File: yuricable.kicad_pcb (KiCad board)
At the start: 2 copper layers, 66.2 x 29.2 mm, 34 parts, among them U1 FlipperZero

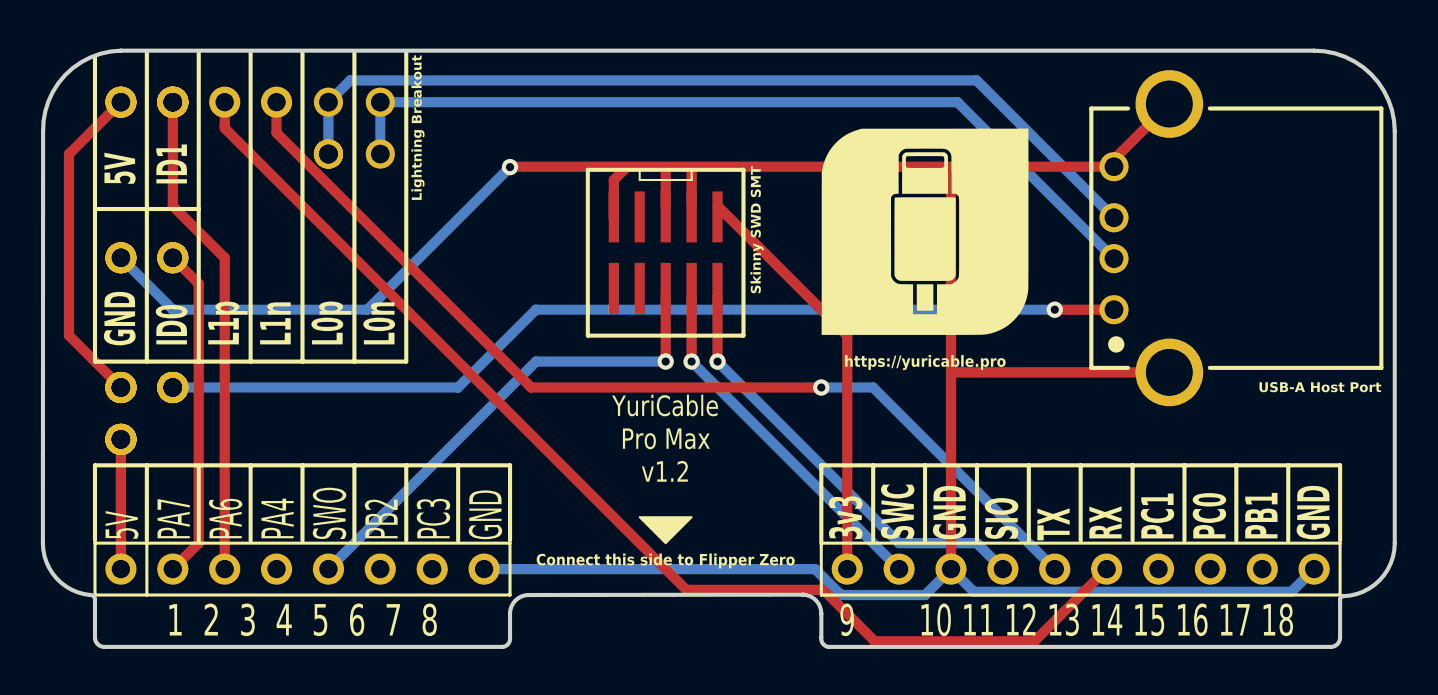
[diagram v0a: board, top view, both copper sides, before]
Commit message: v1.3
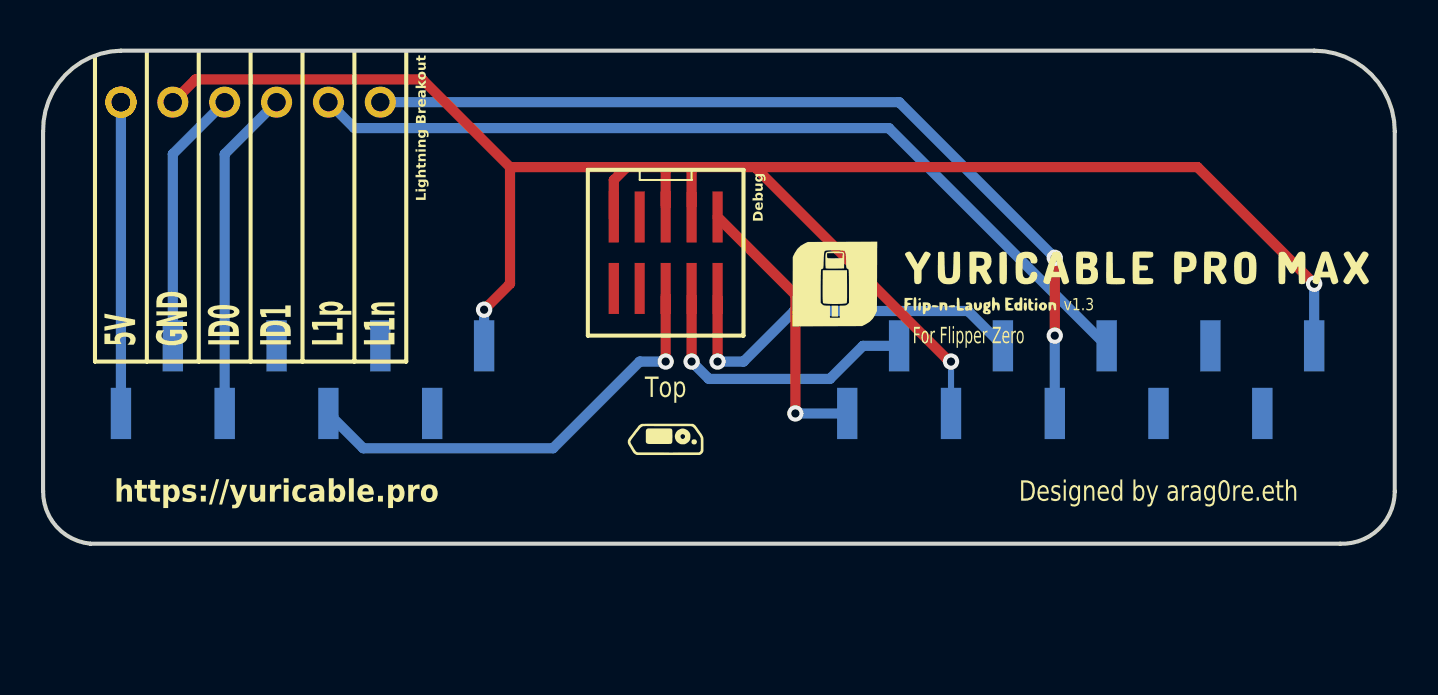
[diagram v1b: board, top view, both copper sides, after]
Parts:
- removed the ? at (66.0, 61.0)
- removed the ? at (66.0, 67.3) (x4)
- removed the ? at (73.7, 53.3)
- removed the ? at (66.0, 53.3) (x3)
- removed the ? at (63.5, 67.3) (x4)
- removed the ? at (76.2, 53.3)
- removed the ? at (73.7, 55.9) (x2)
- removed the ? at (63.5, 61.0)
- removed the ? at (63.5, 69.8) (x4)
- removed the ? at (76.2, 55.9)
- removed the G*** at (102.9, 59.7)
- removed the G*** at (92.7, 61.0)
- removed the REF** at (118.1, 60.0)
- removed U1: FlipperZero, lomalkin_kicad_footprints:FlipperZero
- added 1x8Pins: PinHeader_1x08_P2.54mm_Vertical_SMD_Pin1Left, Connector_PinHeader_2.54mm:PinHeader_1x08_P2.54mm_Vertical_SMD_Pin1Left, F.Cu at (72.4, 66.9)
- added G***: LOGO, YuriCable:Untitled, F.Cu at (110.5, 62.2)
- added G***: LOGO, YuriCable:Untitled, F.Cu at (90.2, 69.8)
- added G***: LOGO, YuriCable:Untitled, B.Cu at (90.2, 69.8)
- added REF**: PinHeader_1x10_P2.54mm_Vertical_SMD_Pin1Left, Connector_PinHeader_2.54mm:PinHeader_1x10_P2.54mm_Vertical_SMD_Pin1Left, F.Cu at (110.5, 66.9)
- moved ? 8.03 mm to (66.0, 53.3)
- moved ? 8.03 mm to (68.6, 53.3)
- moved ? 5.08 mm to (71.1, 53.3)
- moved ? 5.08 mm to (76.2, 53.3)
- moved ? 5.08 mm to (73.7, 53.3)
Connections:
- Skinny SWD SMT pad SWCLK: (no net) -> /SWCLK
- Skinny SWD SMT pad SWDIO: (no net) -> /SWDIO
- Skinny SWD SMT pad SWO: (no net) -> /SWO
- Skinny SWD SMT pad VREF: (no net) -> /3.3V
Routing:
- net /5V: track 70.1 -> 15.2 mm, vias 1 -> 0
- net /USB+: track 44.2 -> 0.00 mm
- net /USB-: track 41.6 -> 0.00 mm
- net GND: track 136.5 -> 95.5 mm, vias 1 -> 3
- net /UART_RX: track 56.3 -> 43.0 mm
- net /PA6: track 23.9 -> 16.3 mm
- net /3.3V: track 20.4 -> 13.7 mm, vias 0 -> 1
- net /UART_TX: track 48.5 -> 43.8 mm, vias 1 -> 2
- net /PA7: track 16.3 -> 13.0 mm
- net /SWCLK: track 17.6 -> 14.4 mm
- net /SWDIO: track 21.4 -> 18.9 mm
- net /SWO: track 23.9 -> 22.2 mm
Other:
- board size 66.2 x 29.2 mm -> 66.2 x 24.1 mm
- board text added: "18 17 16 15 14 13 12 11 10 9"
- board text added: "8 7 6 5 4 3 2 1"
- board text added: "Bottom"
- board text added: "Debug"
- board text added: "Designed by arag0re.eth"
- board text added: "For Flipper Zero"
- board text added: "Top"
- board text added: "v1.3"
- board text removed: "1 2 3 4 5 6 7 8"
- board text removed: "10 11 12 13 14 15 16 17 18"
- board text removed: "9"
- board text removed: "Connect this side to Flipper Zero"
- board text removed: "L0n"
- board text removed: "L0p"
- board text removed: "USB-A Host Port"
- board text removed: "YuriCable Pro Max v1.2"
